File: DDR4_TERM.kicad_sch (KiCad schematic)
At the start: 35 parts

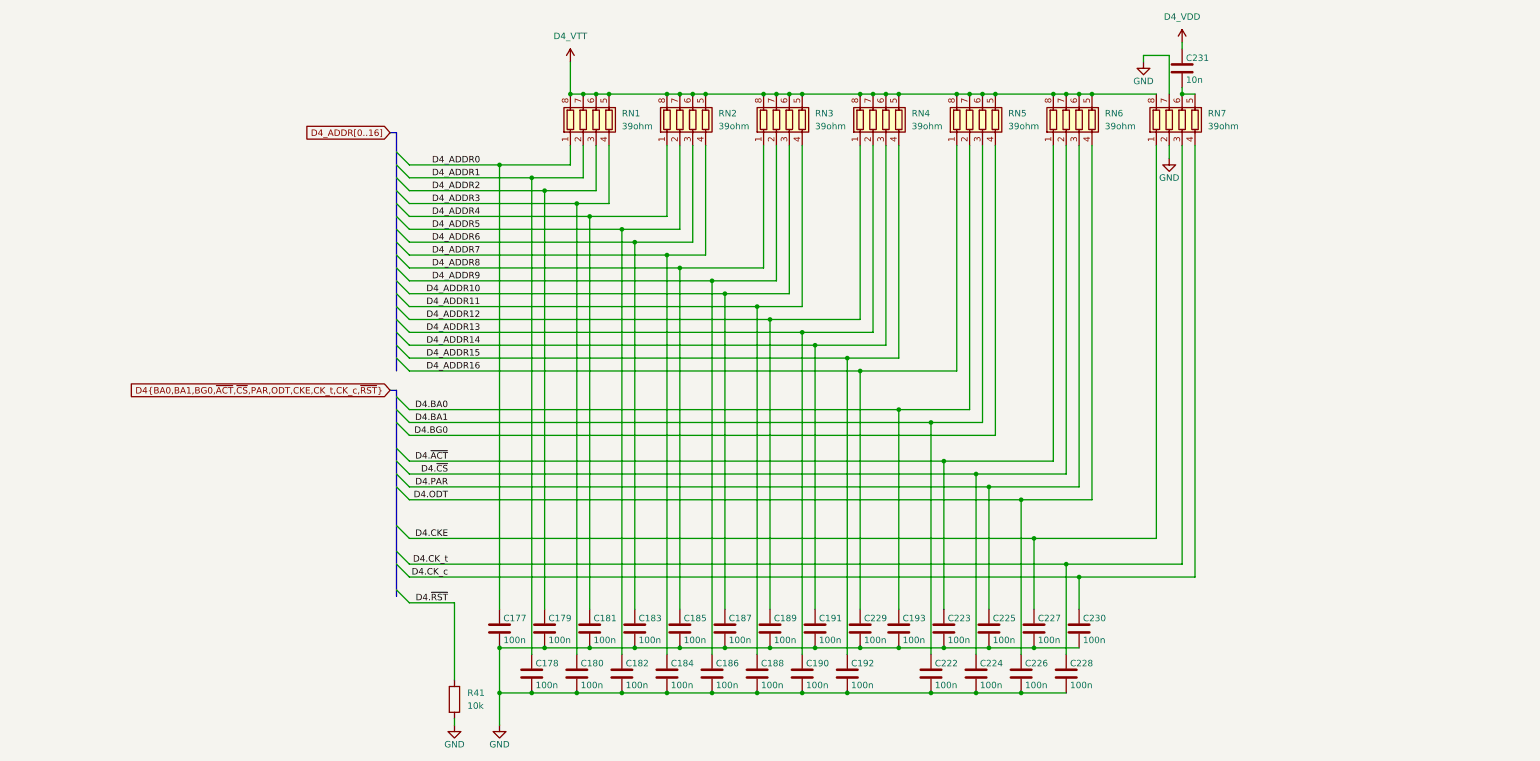
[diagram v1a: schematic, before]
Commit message: sync works
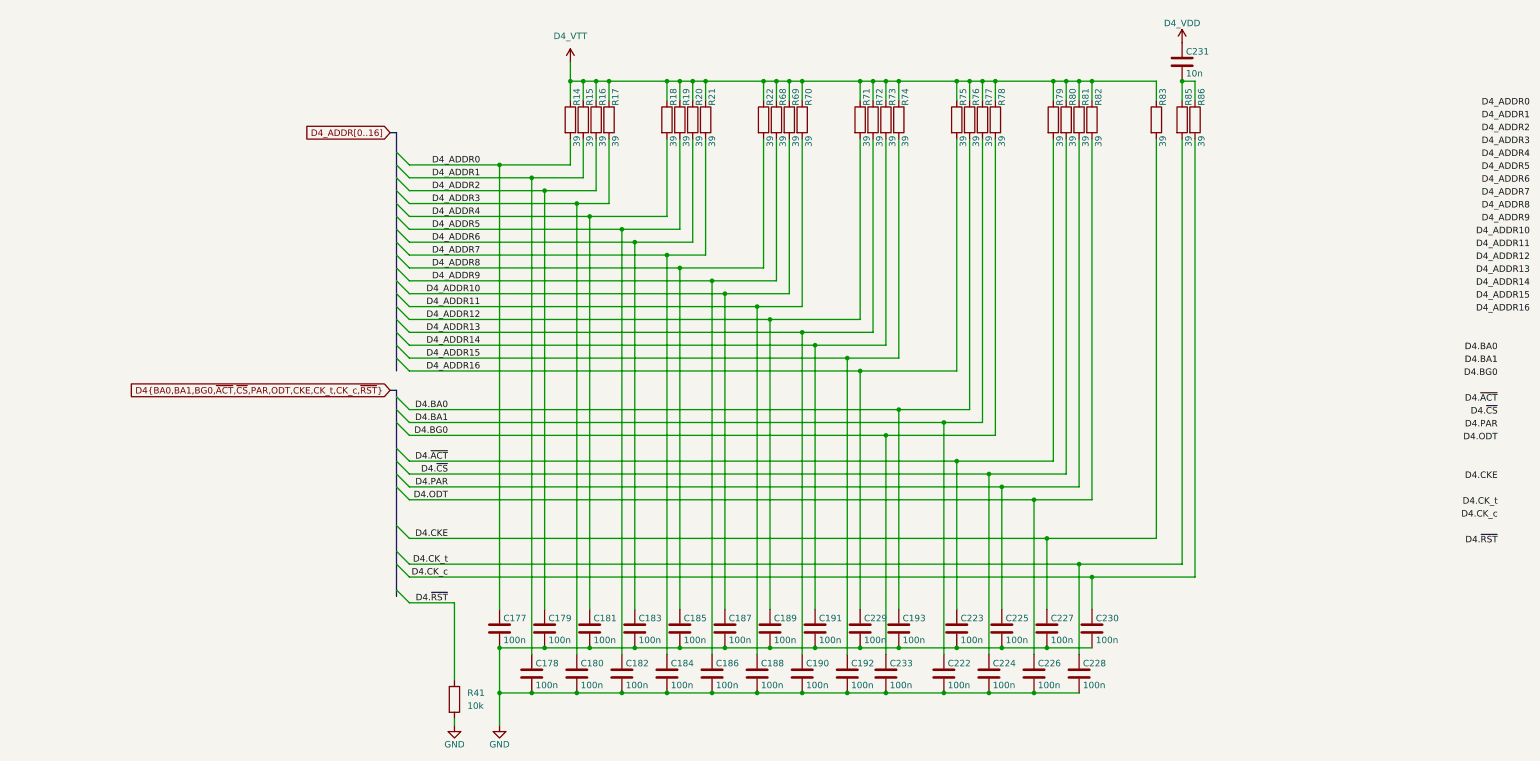
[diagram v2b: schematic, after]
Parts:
- removed RN1, RN2, RN3, RN4, RN5, RN6, RN7: 39ohm, Resistor_SMD:R_Array_Concave_4x0402, symbol Device:R_Pack04
- added C233: 100n, Capacitor_SMD:C_0201_0603Metric, symbol Device:C
- added R14, R15, R16, R17, R18, R19, R20, R21, R22, R68, R69, R70, R71, R72, R73, R74, R75, R76, R77, R78, R79, R80, R81, R82, R83, R85, R86: 39, Resistor_SMD:R_0201_0603Metric, symbol Device:R
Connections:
- net D4.BA0: now also R76.2
- net D4.BA1: now also R77.2
- net D4.BG0: now also C233.1, R78.2
- net D4.CKE: now also R83.2
- net D4.CK_c: now also R86.2
- net D4.CK_t: now also R85.2
- net D4.ODT: now also R82.2
- net D4.PAR: now also R81.2
- net D4.~{ACT}: now also R79.2
- net D4.~{CS}: now also R80.2
- net D4_ADDR0: now also R14.2
- net D4_ADDR1: now also R15.2
- net D4_ADDR10: now also R69.2
- net D4_ADDR11: now also R70.2
- net D4_ADDR12: now also R71.2
- net D4_ADDR13: now also R72.2
- net D4_ADDR14: now also R73.2
- net D4_ADDR15: now also R74.2
- net D4_ADDR16: now also R75.2
- net D4_ADDR2: now also R16.2
- net D4_ADDR3: now also R17.2
- net D4_ADDR4: now also R18.2
- net D4_ADDR5: now also R19.2
- net D4_ADDR6: now also R20.2
- net D4_ADDR7: now also R21.2
- net D4_ADDR8: now also R22.2
- net D4_ADDR9: now also R68.2
- net D4_VTT: now also R14.1, R15.1, R16.1, R17.1, R18.1, R19.1, R20.1, R21.1, R22.1, R68.1, R69.1, R70.1, R71.1, R72.1, R73.1, R74.1, R75.1, R76.1, R77.1, R78.1, R79.1, R80.1, R81.1, R82.1, R83.1
- net GND: now also C233.2
- net at C231.2: now also R85.1, R86.1
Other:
- moved on the sheet: C222, C223, C224, C225, C226, C227, C228, C230, C231
